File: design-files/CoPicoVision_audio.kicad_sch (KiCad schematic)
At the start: 16 parts, among them J501 AudioJack3, U501 SN76489AN, U502 TL071, U503 AY-3-8910, U504 SN74HCT02D

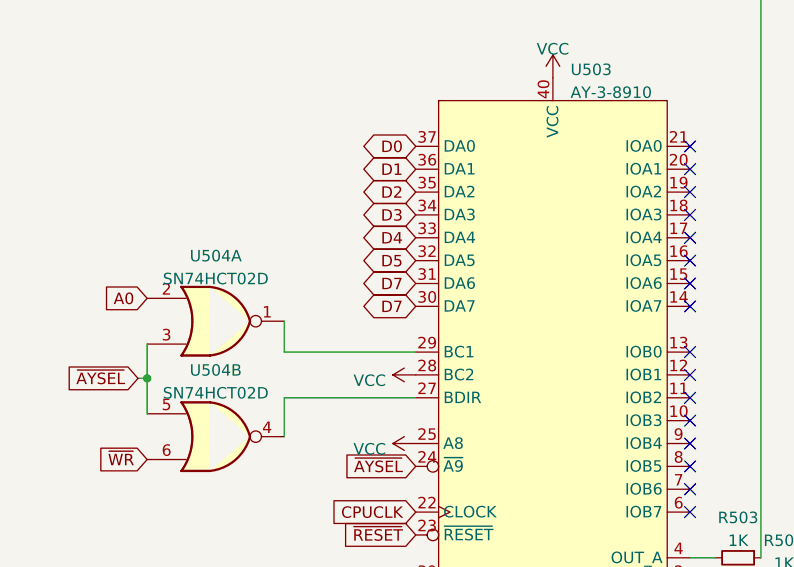
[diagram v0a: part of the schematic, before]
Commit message: I think that's the whole right side of the board now routed.
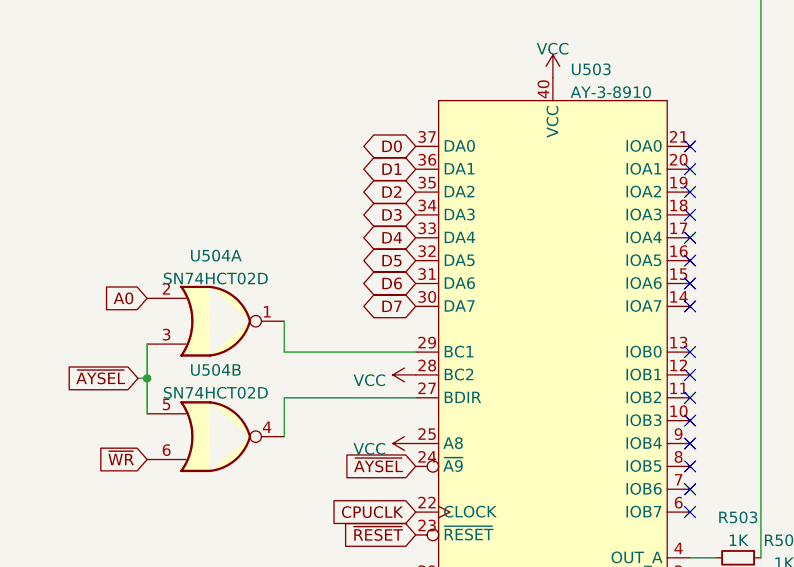
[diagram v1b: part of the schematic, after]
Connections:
- net D6: now also U503.31 (DA6)
- net D7: no longer U503.31 (DA6)
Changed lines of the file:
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@@
     )
   )
-  (global_label "D7" (shape bidirectional) (at 51.181 101.219 180) (fields_autoplaced)
+  (global_label "D6" (shape bidirectional) (at 51.181 101.219 180) (fields_autoplaced)
     (effects (font (size 1.27 1.27)) (justify right))
     (property "Intersheetrefs" "${INTERSHEET_REFS}" (at 44.6844 101.219 0)
